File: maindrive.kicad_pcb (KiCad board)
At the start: 2 copper layers, 112.6 x 130 mm, 15 parts, among them J1 U1_input, J2 U2_input, J3 M1, J4 M2, J5 M3, J6 M4, J7 Encd_sig, J8 Screw_Terminal_01x02, SW1 SW_SPDT, U1 TB6612FNG_Module, U2 TB6612FNG_Module, U3 L7805

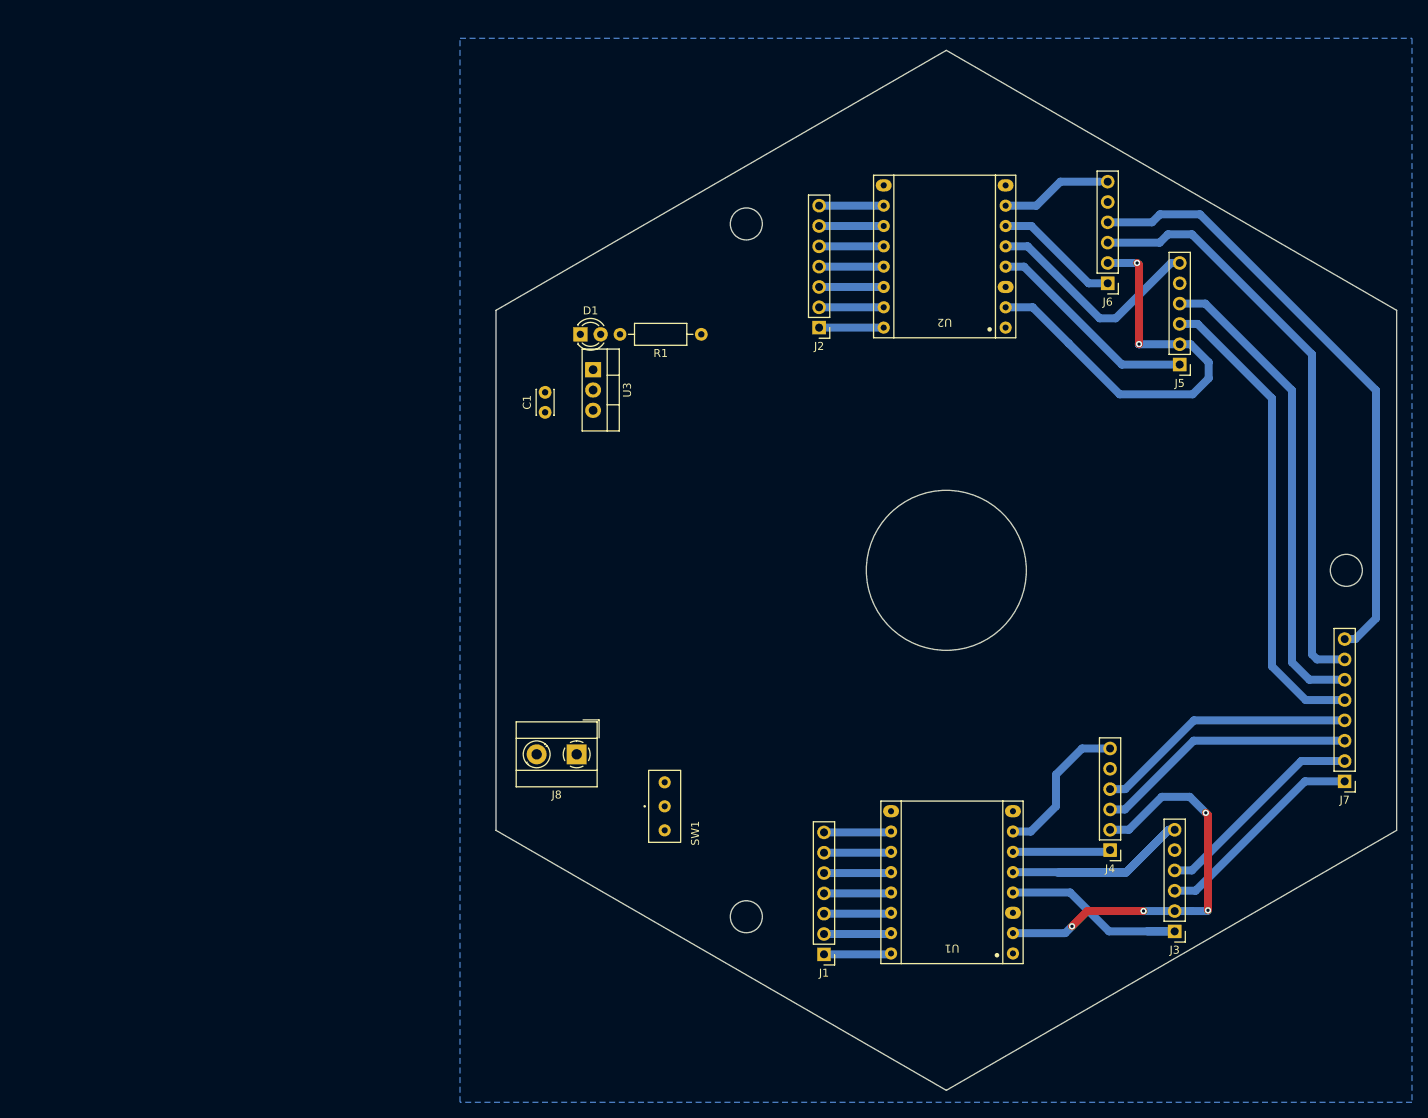
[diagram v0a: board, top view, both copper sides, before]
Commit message: final design
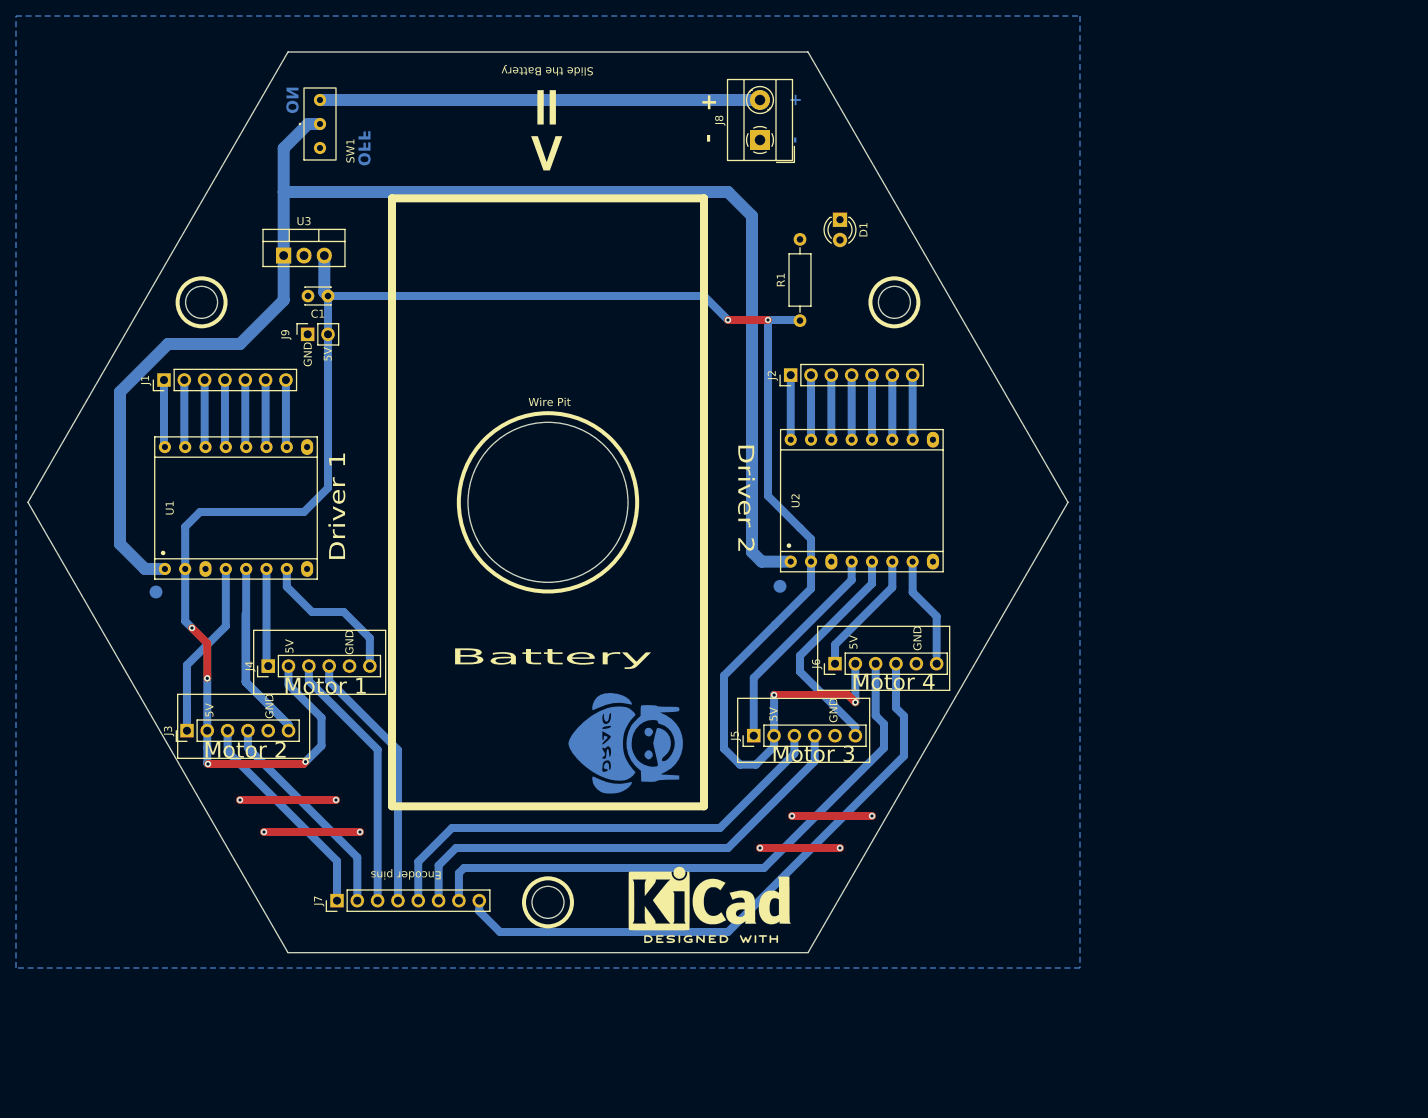
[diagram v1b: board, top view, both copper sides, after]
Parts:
- added G***: LOGO, sche:draic_logo, F.Cu at (111.5, 127.2)
- added J9: Power pins, Connector_PinSocket_2.54mm:PinSocket_1x02_P2.54mm_Vertical, F.Cu at (72.0, 76.0)
- added REF**: KiCad-Logo2_8mm_SilkScreen, Symbol:KiCad-Logo2_8mm_SilkScreen, F.Cu at (122.2, 146.5)
- moved J7 126.8 mm to (75.6, 146.8), turned to 90 degrees
- moved J3 126.0 mm to (56.9, 125.5), turned to 90 degrees
- moved J1 109.4 mm to (54.0, 81.7), turned to 90 degrees
- moved J4 107.7 mm to (67.0, 117.5), turned to 90 degrees
- moved SW1 95.6 mm to (73.5, 49.7)
- moved U1 93.3 mm to (71.9, 105.3), turned to 90 degrees
- moved J8 80.1 mm to (128.5, 51.7), turned to 90 degrees
- moved J5 70.6 mm to (127.7, 126.2), turned to 90 degrees
- moved J6 58.5 mm to (137.9, 117.2), turned to 90 degrees
- moved U2 47.9 mm to (150.1, 104.4), turned to 90 degrees
- moved U3 41.2 mm to (69.0, 66.2), turned to 0 degrees
- moved D1 35.5 mm to (138.5, 61.7), turned to -90 degrees
- moved C1 30.8 mm to (74.5, 71.2), turned to 180 degrees
- moved R1 12.5 mm to (133.5, 74.3), turned to 90 degrees
- moved J2 6.92 mm to (132.3, 81.1), turned to 90 degrees
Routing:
- net VS: track 0.00 -> 183.0 mm
- net +5V: track 108.7 -> 257.2 mm, vias 6 -> 8
- net VCC: track 0.00 -> 55.0 mm
- net GND: track 0.00 -> 44.0 mm, vias 0 -> 8
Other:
- board size 112.6 x 130 mm -> 130 x 112.6 mm
- board text added: "+"
- board text added: "-"
- board text added: "5V"
- board text added: "=>"
- board text added: "Battery"
- board text added: "Designers Note :"
- board text added: "Driver 1"
- board text added: "Driver 2"
- board text added: "Encoder pins"
- board text added: "GND"
- board text added: "Motor 1"
- board text added: "Motor 2"
- board text added: "Motor 3"
- board text added: "Motor 4"
- board text added: "OFF"
- board text added: "ON"
- board text added: "Slide the Battery"
- board text added: "Wire Pit"
